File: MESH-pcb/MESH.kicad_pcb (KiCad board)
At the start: 2 copper layers, 68 parts, among them J1 Ant., J10 USB_C_Receptacle_USB2.0_16P, J12 Conn_01x03_Pin, J2 Conn_01x08_Pin, J3 Conn_01x08_Pin, J4 Conn_01x08_Pin, J5 Conn_01x08_Pin, J6 Conn_01x05_Pin, J7 Conn_01x04_Pin, J8 Conn_01x02, J9 Conn_01x04_Pin, Q1 NMOS, Q2 AO3401A, SW1 SW_Push, SW2 SW_Push, U1 TP4056, U2 CC1101RTK, U4 AP2127R-3.3, U5 STM32L053R8Tx, U6 AP2127R-3.3, Y1 XTM32027000QT00351001, Y2 XTM32027000QT00351001

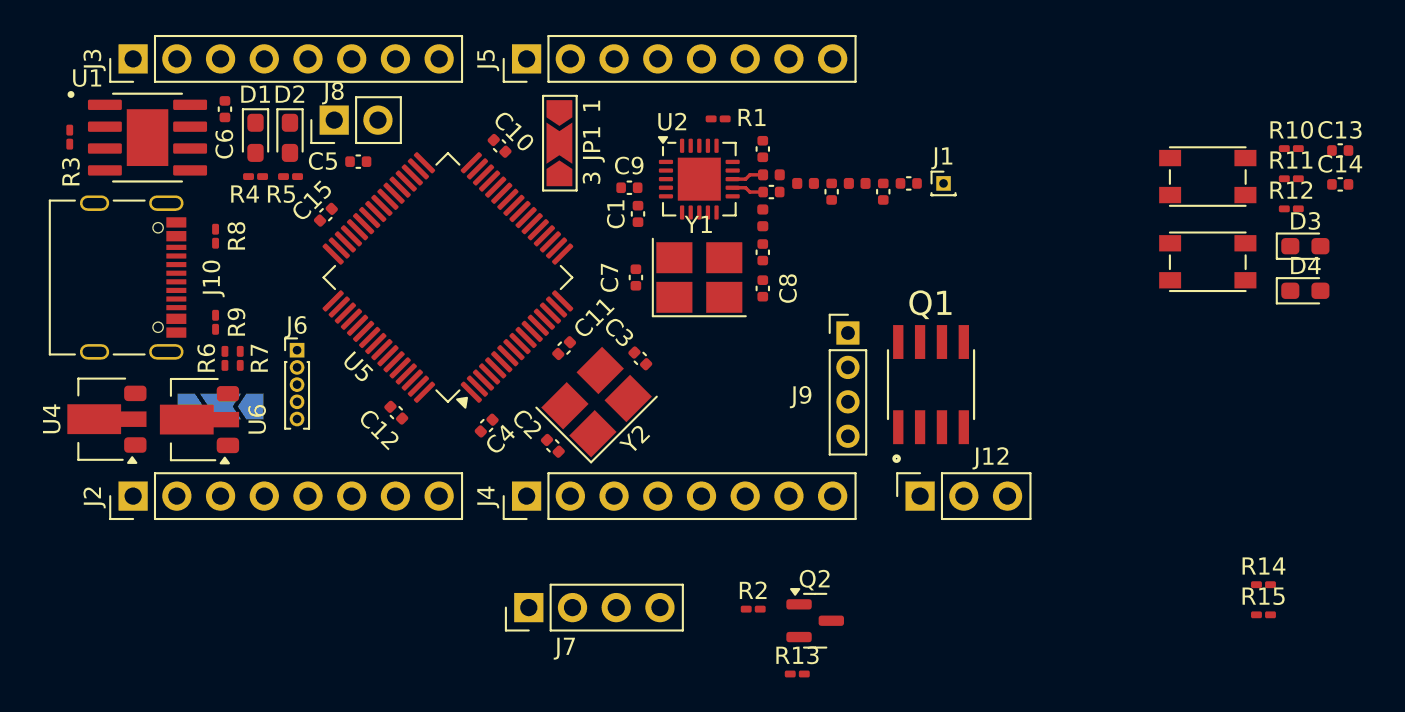
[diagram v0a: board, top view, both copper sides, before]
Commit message: routing almost complete
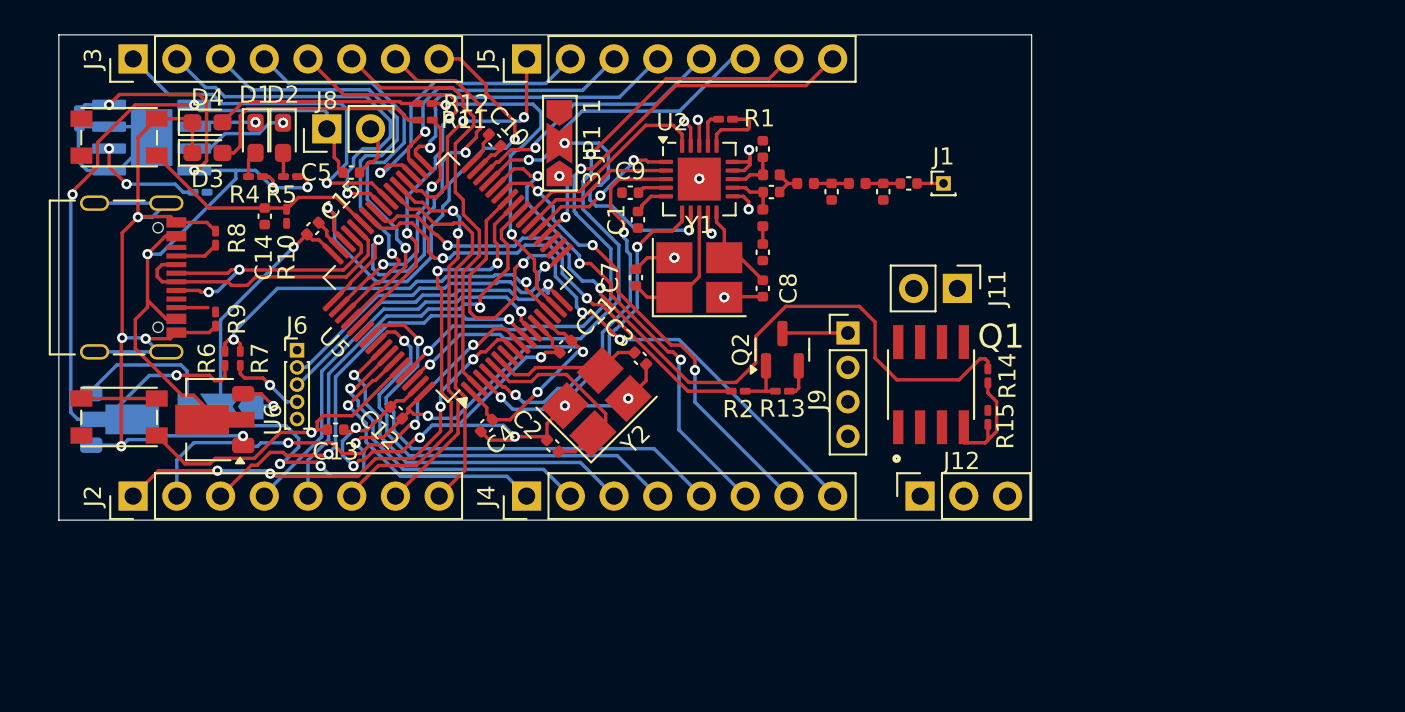
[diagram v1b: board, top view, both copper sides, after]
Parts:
- removed J7: Conn_01x04_Pin, Connector_PinHeader_2.54mm:PinHeader_1x04_P2.54mm_Vertical
- added J11: Conn_01x02_Pin, Connector_PinHeader_2.54mm:PinHeader_1x02_P2.54mm_Vertical, F.Cu at (148.6, 73.5)
- C6, R3, U1, U4: moved to B.Cu
- moved SW1 64.8 mm to (99.8, 81.0)
- moved D4 64.5 mm to (105.0, 63.9)
- moved D3 64.0 mm to (105.0, 65.7)
- moved SW2 63.7 mm to (99.8, 64.8)
- moved C14 62.5 mm to (108.4, 69.3), turned to -90 degrees
- moved C13 60.6 mm to (112.5, 81.7)
- moved R10 58.5 mm to (109.6, 69.3), turned to 90 degrees
- moved R12 50.7 mm to (117.7, 62.8), turned to 180 degrees
- moved R11 50.4 mm to (117.7, 63.8), turned to 180 degrees
- moved R14 20.1 mm to (150.4, 78.6), turned to 90 degrees
- moved R15 19.7 mm to (150.4, 81.0), turned to 90 degrees
- moved R13 16.5 mm to (138.4, 79.5)
- moved Q2 15.9 mm to (138.4, 77.1), turned to 90 degrees
- moved R2 12.7 mm to (135.9, 79.5), turned to 180 degrees
- moved C6 8.48 mm to (97.6, 63.7), turned to -90 degrees
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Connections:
- J3 pad 7: VCC -> /SWCLK
- J3 pad 8: GND -> /SWDIO
- J4 pad 1: unconnected-(J4-Pin_1-Pad1) -> Net-(J4-Pin_1)
- J4 pad 2: unconnected-(J4-Pin_2-Pad2) -> Net-(J4-Pin_2)
- R2 pad 2: /RX2 -> Net-(U5-PA9)
- U1 pad 9: unconnected-(U1-EP-Pad9) -> GND
- U5 pad 42: unconnected-(U5-PA9-Pad42) -> Net-(U5-PA9)
- U5 pad 58: /I2C1_SCL -> Net-(J4-Pin_2)
- U5 pad 59: /I2C1_SDA -> Net-(J4-Pin_1)
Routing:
- net GND: track 0.00 -> 137.8 mm, vias 0 -> 17
- net VCC: track 0.00 -> 68.5 mm, vias 0 -> 10
- net /CTRL: track 0.00 -> 47.7 mm, vias 0 -> 2
- net /charger/Vcc: track 0.00 -> 47.3 mm, vias 0 -> 5
- net /charger/BAT: track 0.00 -> 44.9 mm, vias 0 -> 3
- net Net-(J5-Pin_8): track 0.00 -> 39.8 mm, vias 0 -> 2
- net Net-(J4-Pin_8): track 0.00 -> 37.9 mm, vias 0 -> 3
- net Net-(J5-Pin_7): track 0.00 -> 37.5 mm, vias 0 -> 2
- net Net-(J4-Pin_5): track 0.00 -> 29.2 mm, vias 0 -> 1
- net /SWDIO: track 0.00 -> 28.4 mm, vias 0 -> 2
- net Net-(J4-Pin_6): track 0.00 -> 27.8 mm, vias 0 -> 3
- net Net-(J2-Pin_1): track 0.00 -> 27.7 mm, vias 0 -> 4
- net Net-(J4-Pin_7): track 0.00 -> 27.1 mm, vias 0 -> 3
- net Net-(U5-PA9): track 0.00 -> 27.0 mm, vias 0 -> 2
- net Net-(J2-Pin_2): track 0.00 -> 27.0 mm, vias 0 -> 3
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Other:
- board outline added: 56.5 x 28.2 mm
